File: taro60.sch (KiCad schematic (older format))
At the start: 144 parts, among them SW1 SW_Push, U1 ATmega32U4-AU, Y1 16MHz

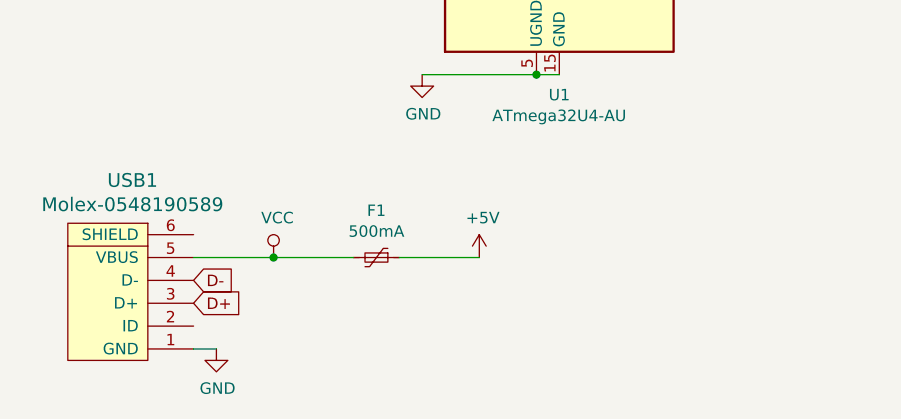
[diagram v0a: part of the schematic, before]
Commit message: updated pcb
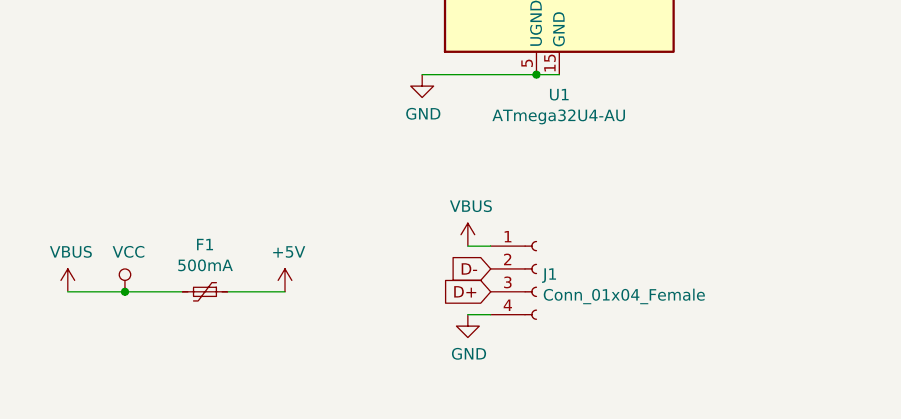
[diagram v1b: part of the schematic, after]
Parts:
- removed USB1: Molex-0548190589, random-keyboard-parts:Molex-0548190589, symbol random-keyboard-parts:Molex-0548190589
- added J1: Conn_01x04_Female, Connector_Molex:Molex_CLIK-Mate_502382-0470_1x04-1MP_P1.25mm_Vertical, symbol Connector:Conn_01x04_Female
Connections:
- net D+: now also J1.3 (Pin_3)
- net D-: now also J1.2 (Pin_2)
- net GND: now also J1.4 (Pin_4)
- net VCC renamed VBUS
- net VBUS: now also J1.1 (Pin_1)
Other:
- moved on the sheet: F1
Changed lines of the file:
@@
 D-
-$Comp
-L random-keyboard-parts:Molex-0548190589 USB1
-U 1 1 6A56638A
-P 1000 7250
-F 0 "USB1" V 1537 7217 60  0000 C CNN
-F 1 "Molex-0548190589" V 1431 7217 60  0000 C CNN
-F 2 "random-keyboard-parts:Molex-0548190589" H 1000 7250 60  0001 C CNN
-F 3 "" H 1000 7250 60  0001 C CNN
-	1    1000 7250
-	0    -1   -1   0
-$EndComp
 $Comp
 L power:VCC #PWR0111
 U 1 1 6A56920F
-P 1650 7050
-F 0 "#PWR0111" H 1650 6900 50  0001 C CNN
-F 1 "VCC" H 1667 7223 50  0000 C CNN
-F 2 "" H 1650 7050 50  0001 C CNN
-F 3 "" H 1650 7050 50  0001 C CNN
-	1    1650 7050
+P 1000 7200
+F 0 "#PWR0111" H 1000 7050 50  0001 C CNN
+F 1 "VCC" H 1017 7373 50  0000 C CNN
+F 2 "" H 1000 7200 50  0001 C CNN
+F 3 "" H 1000 7200 50  0001 C CNN
+	1    1000 7200
 	1    0    0    -1
 $EndComp
@@
 L Device:Polyfuse_Small F1
 U 1 1 6A569F04
-P 2100 7050
-F 0 "F1" V 1895 7050 50  0000 C CNN
-F 1 "500mA" V 1986 7050 50  0000 C CNN
-F 2 "Fuse:Fuse_1206_3216Metric" H 2150 6850 50  0001 L CNN
-F 3 "~" H 2100 7050 50  0001 C CNN
-	1    2100 7050
+P 1350 7200
+F 0 "F1" V 1145 7200 50  0000 C CNN
+F 1 "500mA" V 1236 7200 50  0000 C CNN
+F 2 "Fuse:Fuse_1206_3216Metric" H 1400 7000 50  0001 L CNN
+F 3 "~" H 1350 7200 50  0001 C CNN
+	1    1350 7200
 	0    1    1    0
 $EndComp
@@
 L power:+5V #PWR0112
 U 1 1 6A56A739
-P 2550 7050
-F 0 "#PWR0112" H 2550 6900 50  0001 C CNN
-F 1 "+5V" H 2565 7223 50  0000 C CNN
-F 2 "" H 2550 7050 50  0001 C CNN
-F 3 "" H 2550 7050 50  0001 C CNN
-	1    2550 7050
-	1    0    0    -1
-$EndComp
-Wire Wire Line
-	1300 7050 1650 7050
-Wire Wire Line
-	1650 7050 2000 7050
-Connection ~ 1650 7050
-Wire Wire Line
-	2200 7050 2550 7050
-Text GLabel 1300 7250 2    50   Input ~ 0
+P 1700 7200
+F 0 "#PWR0112" H 1700 7050 50  0001 C CNN
+F 1 "+5V" H 1715 7373 50  0000 C CNN
+F 2 "" H 1700 7200 50  0001 C CNN
+F 3 "" H 1700 7200 50  0001 C CNN
+	1    1700 7200
+	1    0    0    -1
+$EndComp
+Text GLabel 2600 7200 0    50   Input ~ 0
 D+
-Text GLabel 1300 7150 2    50   Input ~ 0
+Text GLabel 2600 7100 0    50   Input ~ 0
 D-
 Wire Wire Line
-	1300 7450 1400 7450
+	2500 7300 2600 7300
 $Comp
 L power:GND #PWR0113
 U 1 1 6A56EF62
-P 1400 7450
-F 0 "#PWR0113" H 1400 7200 50  0001 C CNN
-F 1 "GND" H 1405 7277 50  0000 C CNN
-F 2 "" H 1400 7450 50  0001 C CNN
-F 3 "" H 1400 7450 50  0001 C CNN
-	1    1400 7450
+P 2500 7300
+F 0 "#PWR0113" H 2500 7050 50  0001 C CNN
+F 1 "GND" H 2505 7127 50  0000 C CNN
+F 2 "" H 2500 7300 50  0001 C CNN
+F 3 "" H 2500 7300 50  0001 C CNN
+	1    2500 7300
 	1    0    0    -1
 $EndComp
@@
 Text GLabel 10800 950  1    50   Input ~ 0
 COL13
-Wire Wire Line
-	9000 1950 9000 2650
 Text GLabel 3500 2950 2    50   Input ~ 0
 ROW4
@@
 Text GLabel 3500 5750 2    50   Input ~ 0
 COL13
+$Comp
+L Connector:Conn_01x04_Female J1
+U 1 1 6A546F04
+P 2800 7100
+F 0 "J1" H 2828 7076 50  0000 L CNN
+F 1 "Conn_01x04_Female" H 2828 6985 50  0000 L CNN
+F 2 "Connector_Molex:Molex_CLIK-Mate_502382-0470_1x04-1MP_P1.25mm_Vertical" H 2800 7100 50  0001 C CNN
+F 3 "~" H 2800 7100 50  0001 C CNN
+	1    2800 7100
+	1    0    0    -1
+$EndComp
+$Comp
+L power:VBUS #PWR01
+U 1 1 6A56E25A
+P 2500 7000
+F 0 "#PWR01" H 2500 6850 50  0001 C CNN
+F 1 "VBUS" H 2515 7173 50  0000 C CNN
+F 2 "" H 2500 7000 50  0001 C CNN
+F 3 "" H 2500 7000 50  0001 C CNN
+	1    2500 7000
+	1    0    0    -1
+$EndComp
+Wire Wire Line
+	2500 7000 2600 7000
+$Comp
+L power:VBUS #PWR02
+U 1 1 6A57F672
+P 750 7200
+F 0 "#PWR02" H 750 7050 50  0001 C CNN
+F 1 "VBUS" H 765 7373 50  0000 C CNN
+F 2 "" H 750 7200 50  0001 C CNN
+F 3 "" H 750 7200 50  0001 C CNN
+	1    750  7200
+	1    0    0    -1
+$EndComp
+Wire Wire Line
+	750  7200 1000 7200
+Wire Wire Line
+	1000 7200 1250 7200
+Connection ~ 1000 7200
+Wire Wire Line
+	1450 7200 1700 7200
+Wire Wire Line
+	9000 1950 9000 2650
 $EndSCHEMATC
